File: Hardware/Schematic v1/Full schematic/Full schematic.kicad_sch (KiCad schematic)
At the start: 303 parts, among them J1 Conn_01x02_Male, J10 Conn_01x03_Male, J2 Reset, J3 Encoder, J4 Failure LED, J5 Bluetooth, J6 Conn_01x02_Male, J7 Display, J8 Buttons, J9 Conn_01x02_Male, K1 IM43TS, K2 IM43TS, K3 IM43TS, K4 IM43TS, K5 IM43TS, K6 IM43TS, Q1 BC847, Q10 IRLML6402, Q11 BC847, Q12 IRFZ44, Q13 BC847, Q14 IRLML6402, Q15 BC847, Q16 BSS138, Q17 BC847, Q18 IRF610, Q19 BC847, Q2 BC847, Q20 IRLML6402, Q21 BC847, Q22 IRLML6402, Q23 BFS17, Q24 AFT05MS003N, Q3 BC847, Q4 BC847, Q5 BC847, Q6 IRLML6402, Q7 IRF4905, Q8 IRLML6402, Q9 IRLML6402, U1 74LVC2T45DC, U10 ICS501, U11 STM32F103C8Tx, U12 MCP23017_SS, U13 CAT24C256, U2 74LVC2T45DC, U3 AD9835, U4 LM27313XMF, U5 LM2734X, U6 LM2734X, U7 MAX1837EUT33-T, U8 UC3843_SOIC8, U9 AD5245BRJZ10, X1 50MHz, Y1 8MHz, Y2 32768Hz

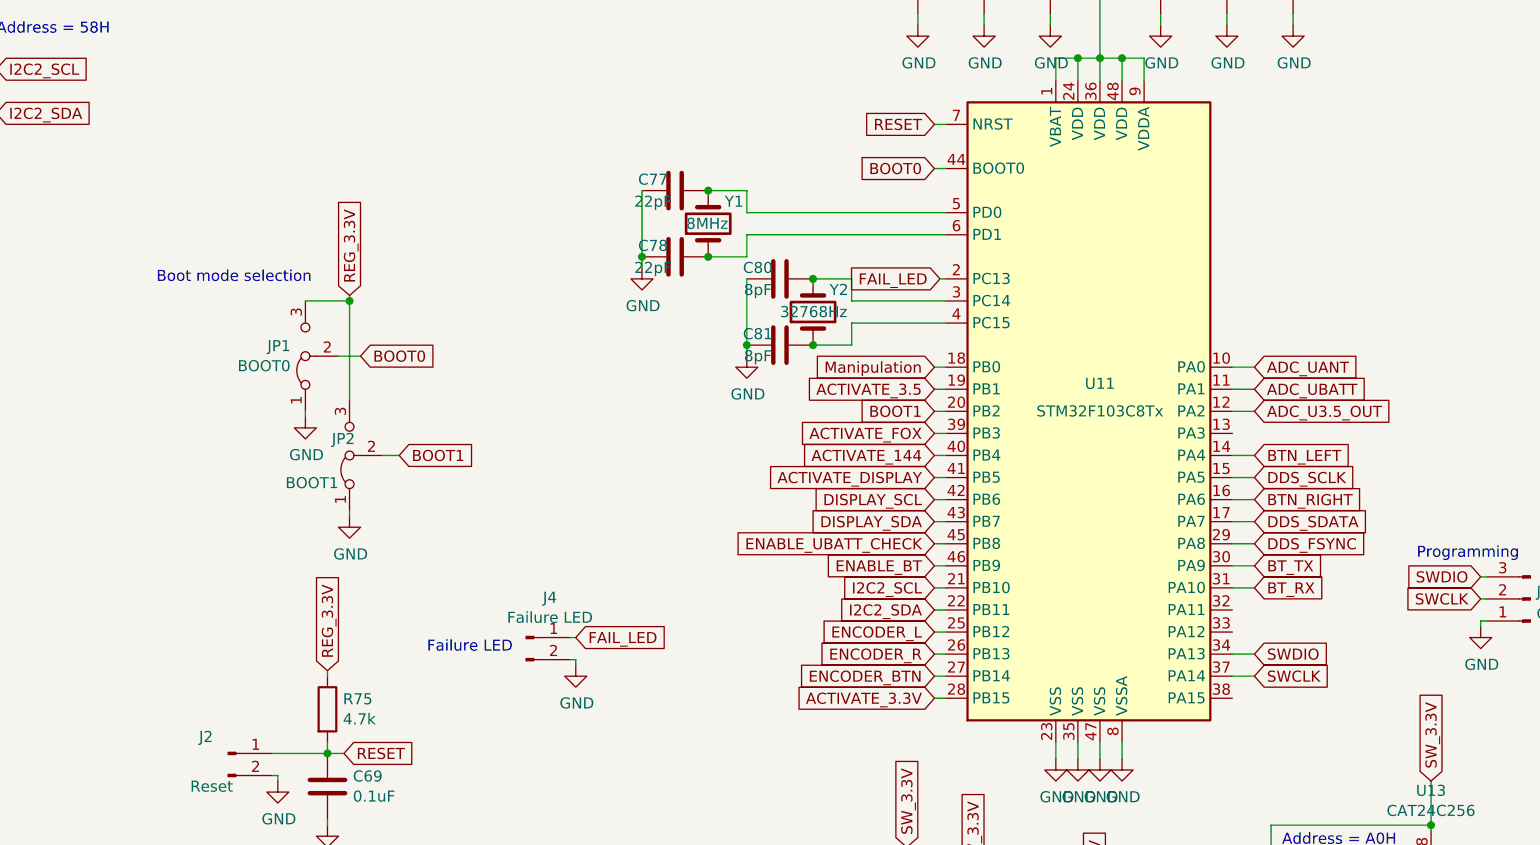
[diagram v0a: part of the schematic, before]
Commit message: PCB tracing is close to an end
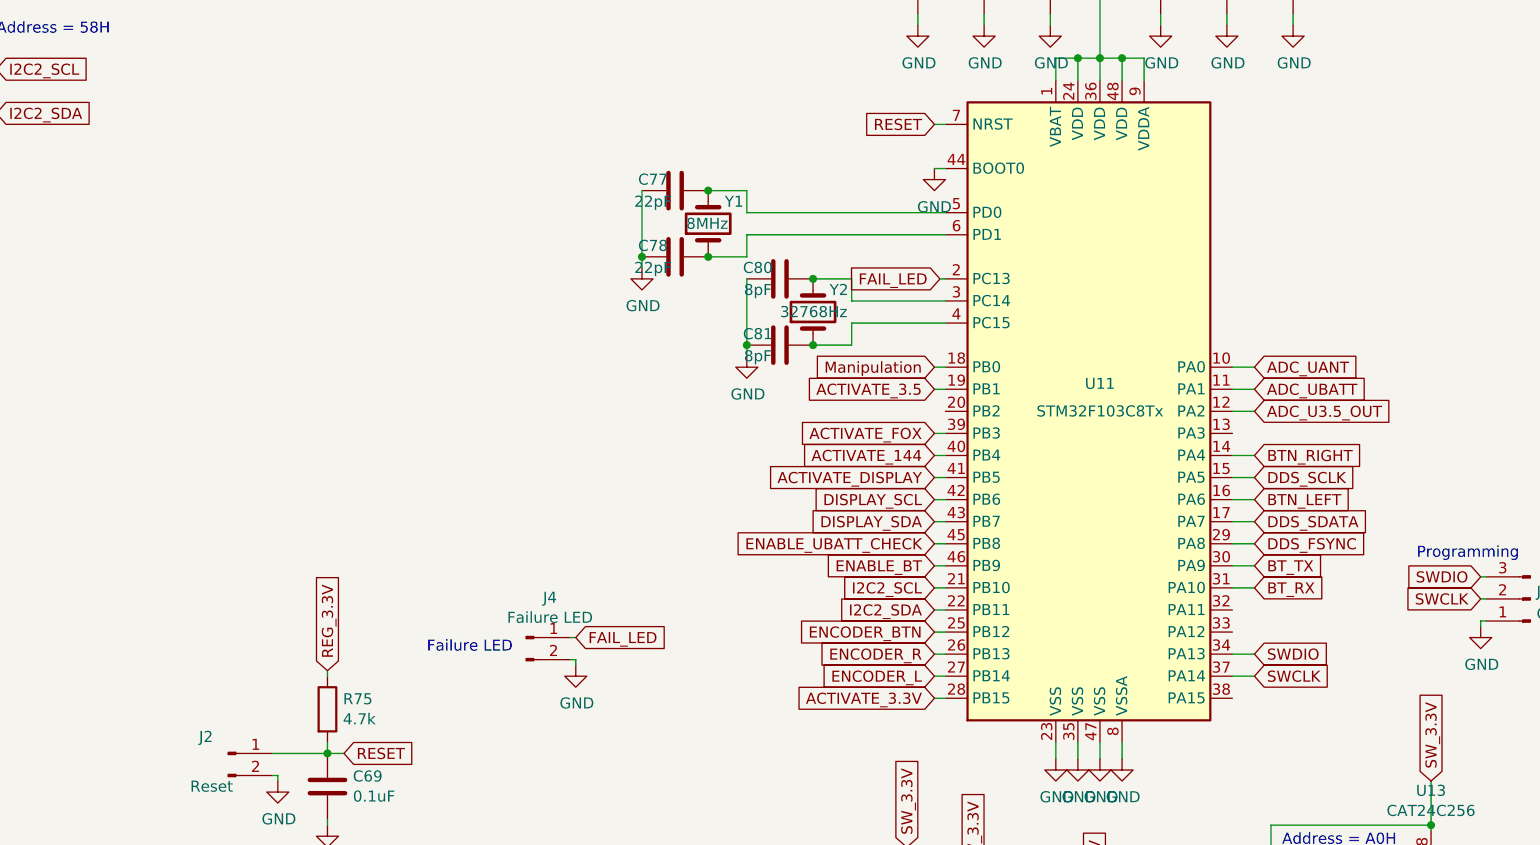
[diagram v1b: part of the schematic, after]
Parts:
- removed JP1: BOOT0, Connector_PinHeader_2.54mm:PinHeader_1x03_P2.54mm_Vertical, symbol Full-schematic-rescue:Jumper_3_Bridged12-Jumper
- removed JP2: BOOT1, Connector_PinHeader_2.54mm:PinHeader_1x03_P2.54mm_Vertical, symbol Full-schematic-rescue:Jumper_3_Bridged12-Jumper
- Y2: footprint Crystal:Crystal_C26-LF_D2.1mm_L6.5mm_Horizontal_1EP_style1 -> Crystal:Crystal_C26-LF_D2.1mm_L6.5mm_Vertical
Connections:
- net BOOT0 is gone; now on net GND: U11.44 (BOOT0)
- net BTN_LEFT: now also U11.16 (PA6); no longer U11.14 (PA4)
- net BTN_RIGHT: now also U11.14 (PA4); no longer U11.16 (PA6)
- net ENCODER_BTN: now also U11.25 (PB12); no longer U11.27 (PB14)
- net ENCODER_L: now also U11.27 (PB14); no longer U11.25 (PB12)
- net BOOT1: no longer names the net of U11.20 (PB2)
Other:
- note removed: "Boot mode selection"
